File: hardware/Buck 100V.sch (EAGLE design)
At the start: 31 parts, among them M1 SI3430DV, M2 SI5435BDC, Q1 FMMT625, Q2 FMMT723, U1 LT3756EMSE

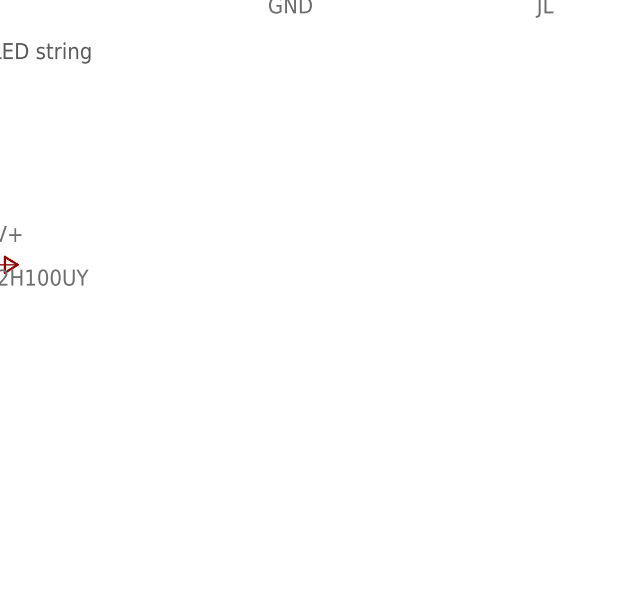
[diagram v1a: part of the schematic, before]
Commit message: Missed from previous commit.
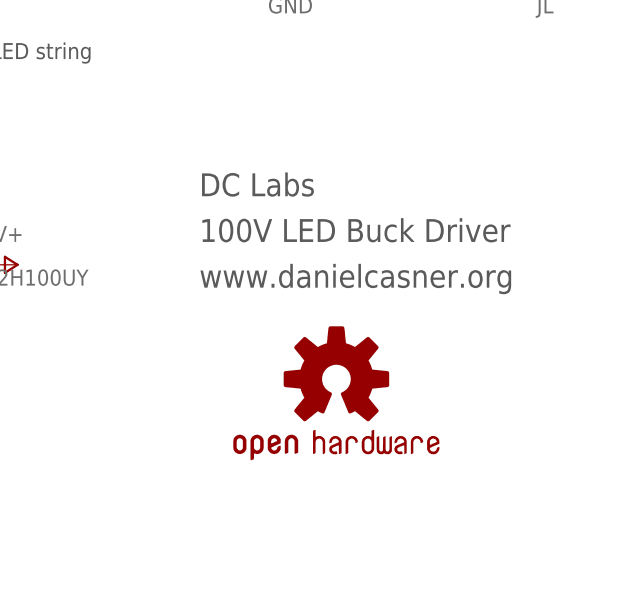
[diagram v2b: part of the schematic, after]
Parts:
- added U$1: OSHW-LOGOS, SparkFun-Aesthetics:OSHW-LOGOS
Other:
- note added: "100V LED Buck Driver"
- note added: "DC Labs"
- note added: "www.danielcasner.org"
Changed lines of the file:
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@@
 <layer number="48" name="Document" color="7" fill="1" visible="no" active="no"/>
 <layer number="49" name="Reference" color="7" fill="1" visible="no" active="no"/>
+<layer number="50" name="dxf" color="7" fill="1" visible="no" active="no"/>
 <layer number="51" name="tDocu" color="7" fill="1" visible="no" active="no"/>
 <layer number="52" name="bDocu" color="7" fill="1" visible="no" active="no"/>
+<layer number="53" name="tGND_GNDA" color="7" fill="9" visible="no" active="no"/>
+<layer number="54" name="bGND_GNDA" color="1" fill="9" visible="no" active="no"/>
+<layer number="56" name="wert" color="7" fill="1" visible="no" active="no"/>
 <layer number="91" name="Nets" color="2" fill="1" visible="yes" active="yes"/>
 <layer number="92" name="Busses" color="1" fill="1" visible="yes" active="yes"/>
@@
 <layer number="97" name="Info" color="7" fill="1" visible="yes" active="yes"/>
 <layer number="98" name="Guide" color="6" fill="1" visible="yes" active="yes"/>
+<layer number="100" name="Muster" color="7" fill="1" visible="no" active="no"/>
+<layer number="101" name="Patch_Top" color="12" fill="4" visible="no" active="yes"/>
+<layer number="102" name="Vscore" color="7" fill="1" visible="no" active="yes"/>
+<layer number="103" name="tMap" color="7" fill="1" visible="no" active="yes"/>
+<layer number="104" name="Name" color="16" fill="1" visible="no" active="yes"/>
+<layer number="105" name="tPlate" color="7" fill="1" visible="no" active="yes"/>
+<layer number="106" name="bPlate" color="7" fill="1" visible="no" active="yes"/>
+<layer number="107" name="Crop" color="7" fill="1" visible="no" active="yes"/>
+<layer number="116" name="Patch_BOT" color="9" fill="4" visible="no" active="yes"/>
+<layer number="121" name="_tsilk" color="7" fill="1" visible="no" active="yes"/>
+<layer number="122" name="_bsilk" color="7" fill="1" visible="no" active="yes"/>
+<layer number="125" name="_tNames" color="7" fill="1" visible="no" active="yes"/>
+<layer number="144" name="Drill_legend" color="7" fill="1" visible="no" active="yes"/>
+<layer number="151" name="HeatSink" color="7" fill="1" visible="no" active="yes"/>
+<layer number="200" name="200bmp" color="1" fill="10" visible="no" active="yes"/>
+<layer number="201" name="201bmp" color="2" fill="10" visible="no" active="yes"/>
+<layer number="202" name="202bmp" color="3" fill="10" visible="no" active="yes"/>
+<layer number="203" name="203bmp" color="4" fill="10" visible="no" active="yes"/>
+<layer number="204" name="204bmp" color="5" fill="10" visible="no" active="yes"/>
+<layer number="205" name="205bmp" color="6" fill="10" visible="no" active="yes"/>
+<layer number="206" name="206bmp" color="7" fill="10" visible="no" active="yes"/>
+<layer number="207" name="207bmp" color="8" fill="10" visible="no" active="yes"/>
+<layer number="208" name="208bmp" color="9" fill="10" visible="no" active="yes"/>
+<layer number="209" name="209bmp" color="7" fill="1" visible="no" active="yes"/>
+<layer number="210" name="210bmp" color="7" fill="1" visible="no" active="yes"/>
+<layer number="211" name="211bmp" color="7" fill="1" visible="no" active="yes"/>
+<layer number="212" name="212bmp" color="7" fill="1" visible="no" active="yes"/>
+<layer number="213" name="213bmp" color="7" fill="1" visible="no" active="yes"/>
+<layer number="214" name="214bmp" color="7" fill="1" visible="no" active="yes"/>
+<layer number="215" name="215bmp" color="7" fill="1" visible="no" active="yes"/>
+<layer number="216" name="216bmp" color="7" fill="1" visible="no" active="yes"/>
+<layer number="217" name="217bmp" color="18" fill="1" visible="no" active="no"/>
+<layer number="218" name="218bmp" color="19" fill="1" visible="no" active="no"/>
+<layer number="219" name="219bmp" color="20" fill="1" visible="no" active="no"/>
+<layer number="220" name="220bmp" color="21" fill="1" visible="no" active="no"/>
+<layer number="221" name="221bmp" color="22" fill="1" visible="no" active="no"/>
+<layer number="222" name="222bmp" color="23" fill="1" visible="no" active="no"/>
+<layer number="223" name="223bmp" color="24" fill="1" visible="no" active="no"/>
+<layer number="224" name="224bmp" color="25" fill="1" visible="no" active="no"/>
+<layer number="250" name="Descript" color="3" fill="1" visible="no" active="no"/>
+<layer number="251" name="SMDround" color="12" fill="11" visible="no" active="no"/>
+<layer number="254" name="cooling" color="7" fill="1" visible="no" active="yes"/>
 </layers>
 <schematic xreflabel="%F%N/%S.%C%R" xrefpart="/%S.%C%R">
@@
 <part name="RIS_SMD" library="LED-drivers" deviceset="R-KELVIN" device="R2512"/>
 <part name="RIS_PTH" library="LED-drivers" deviceset="R-KELVIN" device="0204/7"/>
+<part name="U$1" library="SparkFun-Aesthetics" deviceset="OSHW-LOGO" device="S"/>
 </parts>
 <sheets>
@@
 <text x="119.38" y="45.72" size="1.27" layer="97" rot="R90">sense resistor</text>
 <text x="111.76" y="2.54" size="1.778" layer="97">External LED string</text>
+<text x="144.78" y="-12.7" size="2.54" layer="97">DC Labs</text>
+<text x="144.78" y="-17.78" size="2.54" layer="97">100V LED Buck Driver</text>
+<text x="144.78" y="-22.86" size="2.54" layer="97">www.danielcasner.org</text>
 </plain>
 <instances>
@@
 <instance part="RIS_SMD" gate="G$1" x="99.06" y="50.8" rot="R90"/>
 <instance part="RIS_PTH" gate="G$1" x="109.22" y="50.8" rot="R90"/>
+<instance part="U$1" gate="G$1" x="160.02" y="-33.02"/>
 </instances>
 <busses>
